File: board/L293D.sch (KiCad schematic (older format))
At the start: 30 parts, among them J3.1 Conn_01x02, J3.2 Conn_01x02, J3.3 Conn_01x02, J3.4 Conn_01x02, U3.1 L293D, U3.2 L293D

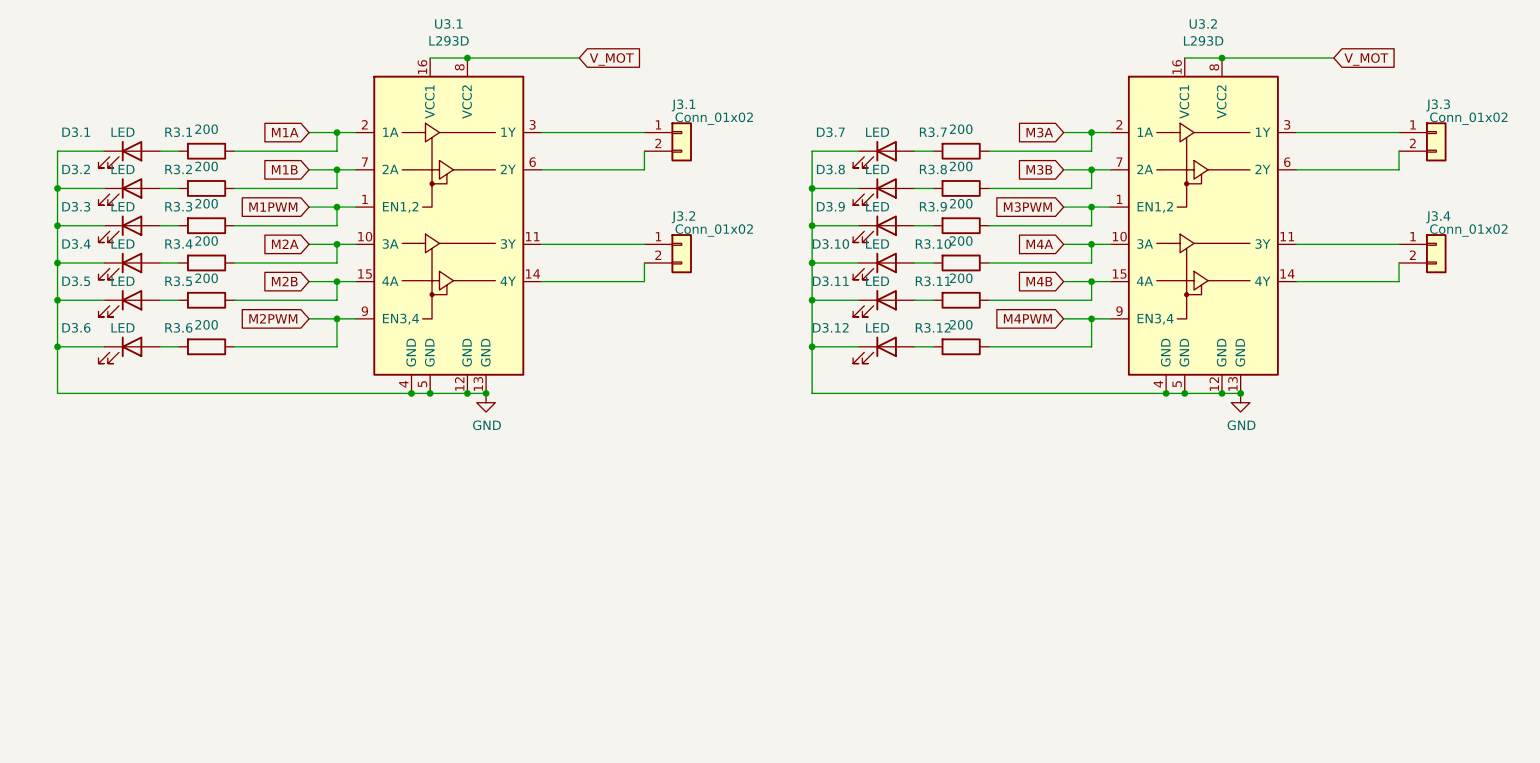
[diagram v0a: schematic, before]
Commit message: updated pcb design
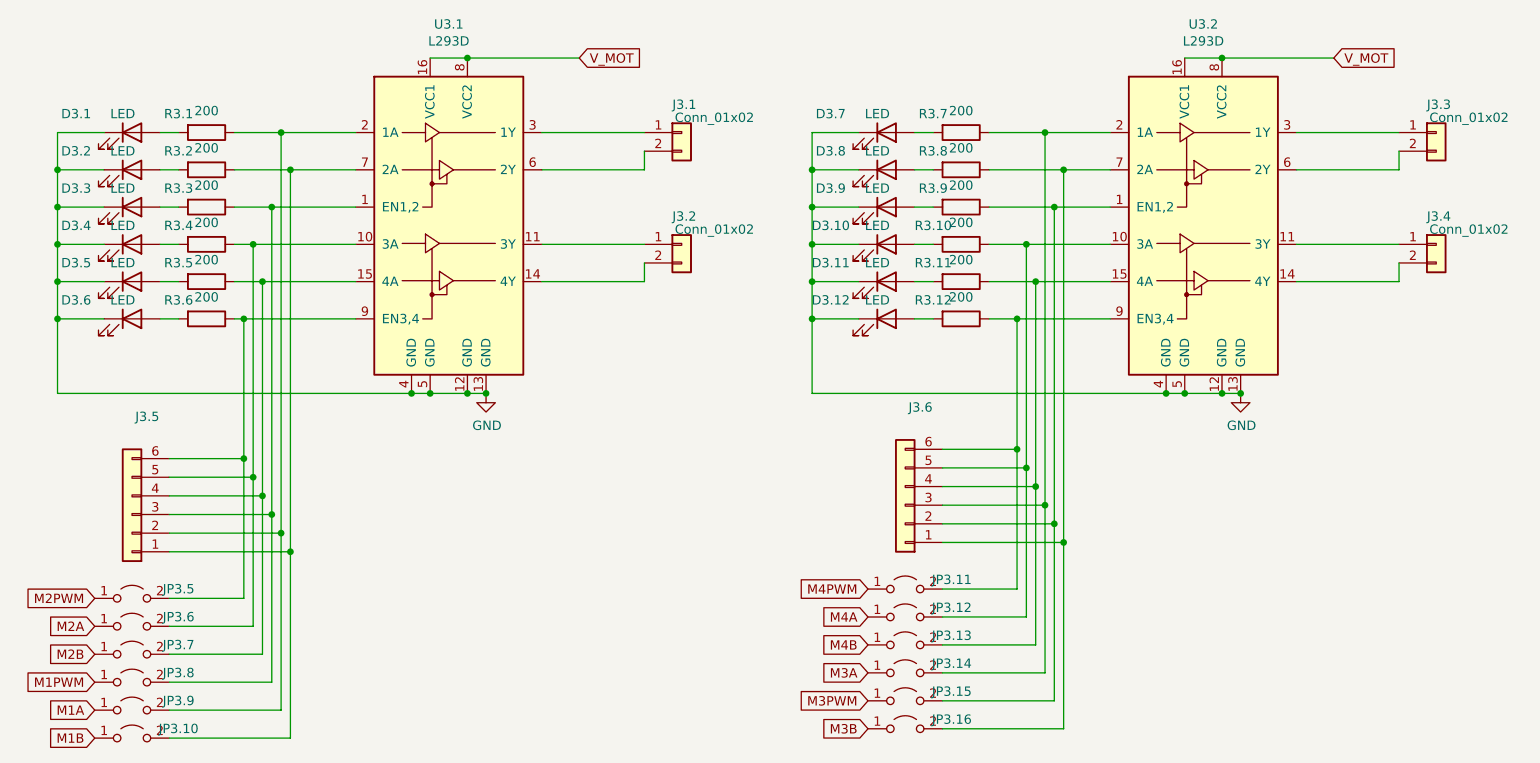
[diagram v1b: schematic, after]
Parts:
- added J3.5, J3.6: Conn_01x06, Connector_PinHeader_2.54mm:PinHeader_1x06_P2.54mm_Vertical, symbol Connector_Generic:Conn_01x06
- added JP3.10: M1B, Jumper:SolderJumper-2_P1.3mm_Open_TrianglePad1.0x1.5mm, symbol Jumper:Jumper_2_Open
- added JP3.11: M4PWM, Jumper:SolderJumper-2_P1.3mm_Open_TrianglePad1.0x1.5mm, symbol Jumper:Jumper_2_Open
- added JP3.12: M4A, Jumper:SolderJumper-2_P1.3mm_Open_TrianglePad1.0x1.5mm, symbol Jumper:Jumper_2_Open
- added JP3.13: M4B, Jumper:SolderJumper-2_P1.3mm_Open_TrianglePad1.0x1.5mm, symbol Jumper:Jumper_2_Open
- added JP3.14: M3A, Jumper:SolderJumper-2_P1.3mm_Open_TrianglePad1.0x1.5mm, symbol Jumper:Jumper_2_Open
- added JP3.15: M3PWM, Jumper:SolderJumper-2_P1.3mm_Open_TrianglePad1.0x1.5mm, symbol Jumper:Jumper_2_Open
- added JP3.16: M3B, Jumper:SolderJumper-2_P1.3mm_Open_TrianglePad1.0x1.5mm, symbol Jumper:Jumper_2_Open
- added JP3.5: M2PWM, Jumper:SolderJumper-2_P1.3mm_Open_TrianglePad1.0x1.5mm, symbol Jumper:Jumper_2_Open
- added JP3.6: M2A, Jumper:SolderJumper-2_P1.3mm_Open_TrianglePad1.0x1.5mm, symbol Jumper:Jumper_2_Open
- added JP3.7: M2B, Jumper:SolderJumper-2_P1.3mm_Open_TrianglePad1.0x1.5mm, symbol Jumper:Jumper_2_Open
- added JP3.8: M1PWM, Jumper:SolderJumper-2_P1.3mm_Open_TrianglePad1.0x1.5mm, symbol Jumper:Jumper_2_Open
- added JP3.9: M1A, Jumper:SolderJumper-2_P1.3mm_Open_TrianglePad1.0x1.5mm, symbol Jumper:Jumper_2_Open
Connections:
- net M1A: now also JP3.9.1 (A); no longer R3.1.1, U3.1.2 (1A)
- net M1B: now also JP3.10.1 (A); no longer R3.2.1, U3.1.7 (2A)
- net M1PWM: now also JP3.8.1 (A); no longer R3.3.1, U3.1.1 (EN1,2)
- net M2A: now also JP3.6.1 (A); no longer R3.4.1, U3.1.10 (3A)
- net M2B: now also JP3.7.1 (A); no longer R3.5.1, U3.1.15 (4A)
- net M2PWM: now also JP3.5.1 (A); no longer R3.6.1, U3.1.9 (EN3,4)
- net M3A: now also JP3.14.1 (A); no longer R3.7.1, U3.2.2 (1A)
- net M3B: now also JP3.16.1 (A); no longer R3.8.1, U3.2.7 (2A)
- net M3PWM: now also JP3.15.1 (A); no longer R3.9.1, U3.2.1 (EN1,2)
- net M4A: now also JP3.12.1 (A); no longer R3.10.1, U3.2.10 (3A)
- net M4B: now also JP3.13.1 (A); no longer R3.11.1, U3.2.15 (4A)
- net M4PWM: now also JP3.11.1 (A); no longer R3.12.1, U3.2.9 (EN3,4)
- new net: J3.5.2 (Pin_2), JP3.9.2 (B), R3.1.1, U3.1.2 (1A)
- new net: J3.5.1 (Pin_1), JP3.10.2 (B), R3.2.1, U3.1.7 (2A)
- new net: J3.5.3 (Pin_3), JP3.8.2 (B), R3.3.1, U3.1.1 (EN1,2)
- new net: J3.5.5 (Pin_5), JP3.6.2 (B), R3.4.1, U3.1.10 (3A)
- new net: J3.5.4 (Pin_4), JP3.7.2 (B), R3.5.1, U3.1.15 (4A)
- new net: J3.5.6 (Pin_6), JP3.5.2 (B), R3.6.1, U3.1.9 (EN3,4)
- new net: J3.6.2 (Pin_2), JP3.15.2 (B), R3.9.1, U3.2.1 (EN1,2)
- new net: J3.6.5 (Pin_5), JP3.12.2 (B), R3.10.1, U3.2.10 (3A)
- new net: J3.6.4 (Pin_4), JP3.13.2 (B), R3.11.1, U3.2.15 (4A)
- new net: J3.6.3 (Pin_3), JP3.14.2 (B), R3.7.1, U3.2.2 (1A)
- new net: J3.6.1 (Pin_1), JP3.16.2 (B), R3.8.1, U3.2.7 (2A)
- new net: J3.6.6 (Pin_6), JP3.11.2 (B), R3.12.1, U3.2.9 (EN3,4)
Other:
- moved on the sheet: D3.1, D3.10, D3.11, D3.12, D3.2, D3.3, D3.4, D3.5, D3.6, D3.7, D3.8, D3.9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
